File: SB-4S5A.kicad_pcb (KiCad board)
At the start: 4 copper layers, 100 x 50 mm, 41 parts, among them J1 Conn_02x03_Top_Bottom, Q1 CSD17308Q3, Q2 CSD17308Q3, Q3 2N7002, U1 bq40z50-r2

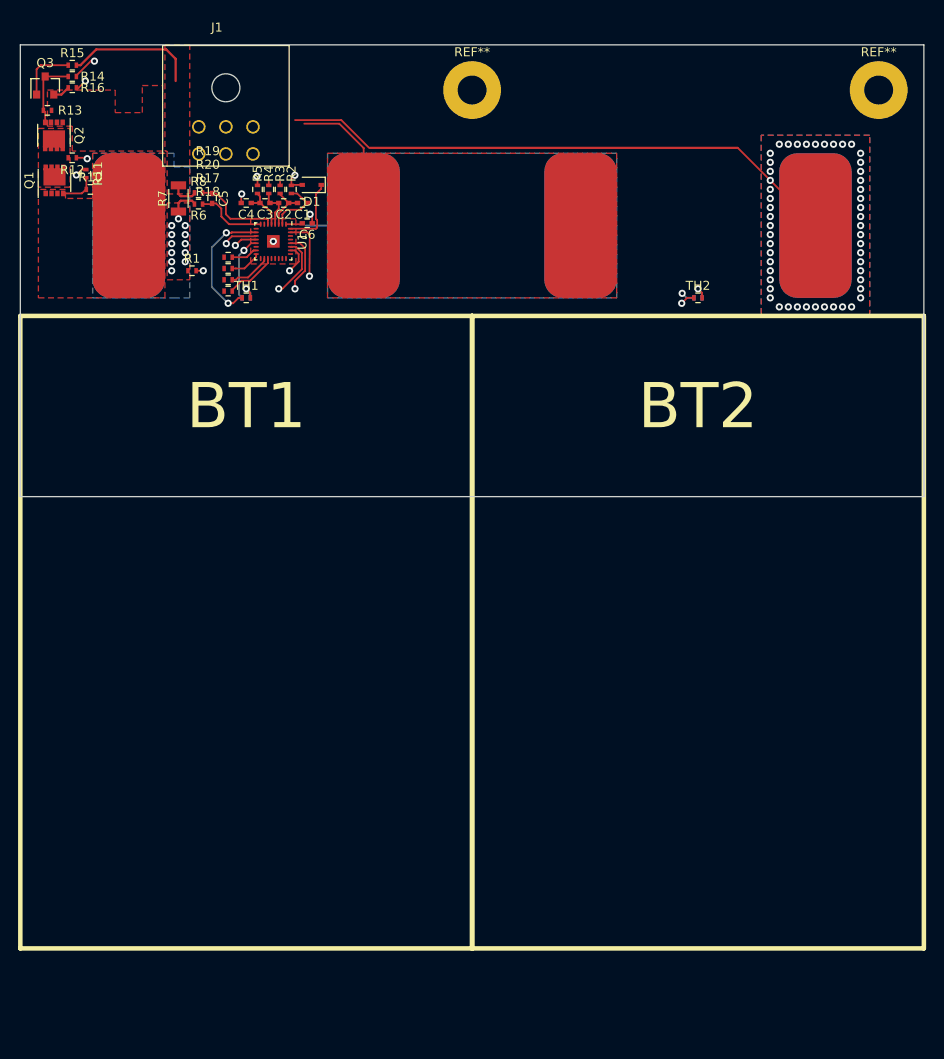
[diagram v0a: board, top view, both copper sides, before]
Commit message: Ready to send to manufacturer.
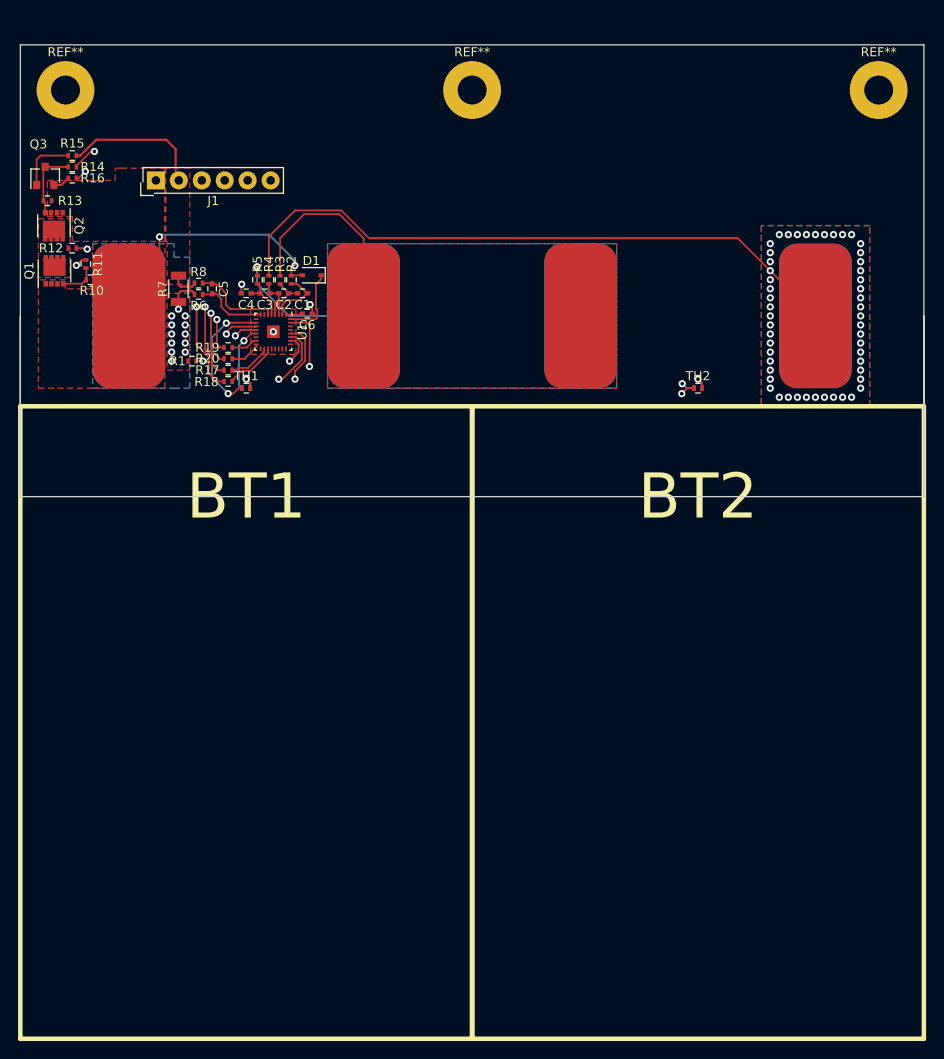
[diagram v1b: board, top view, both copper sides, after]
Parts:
- added REF**: MountingHole_3.2mm_M3_Pad, Mounting_Holes:MountingHole_3.2mm_M3_Pad, F.Cu at (75.0, 65.0)
- J1: value Conn_02x03_Top_Bottom -> LEMO6; footprint Connectors_Molex:Molex_Microfit3_Header_02x03_Angled_43045-060x -> Connectors_Samtec:SL-106-X-XX_1x06
- moved BT1 10.0 mm to (95.0, 100.0)
- moved BT2 10.0 mm to (145.0, 100.0)
- moved BT3 10.0 mm to (145.0, 100.0)
- moved BT4 10.0 mm to (95.0, 100.0)
- moved C1 10.0 mm to (101.2, 87.5)
- moved C2 10.0 mm to (99.2, 87.5)
- moved C3 10.0 mm to (97.1, 87.5)
- moved C4 10.0 mm to (95.0, 87.5)
- moved C5 10.0 mm to (91.2, 87.0)
- moved C6 10.0 mm to (101.8, 89.8)
- moved D1 10.0 mm to (102.2, 85.5)
- moved Q1 10.0 mm to (73.8, 85.0)
- moved Q2 10.0 mm to (73.7, 80.0)
- moved Q3 10.0 mm to (72.8, 74.5)
- moved R1 10.0 mm to (89.0, 95.0)
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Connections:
- U1 pad 17: Net-(U1-Pad17) -> (no net)
- U1 pad 20: Net-(U1-Pad20) -> (no net)
- U1 pad 21: Net-(U1-Pad21) -> (no net)
- U1 pad 22: Net-(U1-Pad22) -> (no net)
- U1 pad 25: Net-(U1-Pad25) -> (no net)
- U1 pad 30: Net-(U1-Pad30) -> (no net)
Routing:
- net /BAT+: track 2.50 -> 29.5 mm, vias 1 -> 2
- net /BTP_INT: track 0.00 -> 24.4 mm, vias 0 -> 1
- net /SMBC: track 0.00 -> 24.2 mm, vias 0 -> 1
- net /~PRES~: track 0.10 -> 23.9 mm, vias 0 -> 1
- net /SMBD: track 0.10 -> 23.3 mm, vias 0 -> 1
- net /VC1A: track 7.42 -> 16.2 mm
- net /VC2A: track 62.9 -> 70.8 mm
- net /VC3A: track 16.7 -> 24.2 mm

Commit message: Fix FUSE pin floating.
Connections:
- U1 pad 25: (no net) -> GNDD
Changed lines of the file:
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@@
   (page A4)
   (layers
-    (0 F.Cu signal hide)
+    (0 F.Cu signal)
     (1 In1.Cu mixed hide)
     (2 In2.Cu mixed hide)
@@
     (pad 24 smd oval (at 1.9 -1.4) (size 0.2 0.6) (layers F.Cu F.Paste F.Mask)
       (net 1 GNDD))
-    (pad 25 smd oval (at 1.4 -1.9 270) (size 0.2 0.6) (layers F.Cu F.Paste F.Mask))
+    (pad 25 smd oval (at 1.4 -1.9 270) (size 0.2 0.6) (layers F.Cu F.Paste F.Mask)
+      (net 1 GNDD))
     (pad 26 smd oval (at 1 -1.9 270) (size 0.2 0.6) (layers F.Cu F.Paste F.Mask)
       (net 30 /_VCC_))
@@
   (segment (start 103.3 85.925) (end 103.3 85.5) (width 0.2) (layer F.Cu) (net 21) (status 20))
   (segment (start 91.2 95.4) (end 91.8 96) (width 0.2) (layer F.Cu) (net 22))
-  (segment (start 91.8 96) (end 92.55 96) (width 0.2) (layer F.Cu) (net 22))
+  (segment (start 91.8 96) (end 92.55 96) (width 0.2) (layer F.Cu) (net 22) (status 20))
   (segment (start 91.2 94.4) (end 91.2 95.4) (width 0.2) (layer F.Cu) (net 22))
   (segment (start 90.45 93.65) (end 91.2 94.4) (width 0.2) (layer F.Cu) (net 22))
   (segment (start 90.45 89) (end 90.45 93.65) (width 0.2) (layer F.Cu) (net 22))
-  (segment (start 92.62 75) (end 90.45 77.17) (width 0.2) (layer In2.Cu) (net 22))
+  (segment (start 92.62 75) (end 90.45 77.17) (width 0.2) (layer In2.Cu) (net 22) (status 10))
   (segment (start 90.45 77.17) (end 90.45 89) (width 0.2) (layer In2.Cu) (net 22))
   (via (at 90.45 89) (size 0.8) (drill 0.4) (layers F.Cu B.Cu) (net 22))
@@
   (segment (start 90.08 88.42) (end 89.5 89) (width 0.2) (layer In2.Cu) (net 23))
   (segment (start 91.1 93.8) (end 92.05 94.75) (width 0.2) (layer F.Cu) (net 24))
-  (segment (start 92.05 94.75) (end 92.55 94.75) (width 0.2) (layer F.Cu) (net 24))
+  (segment (start 92.05 94.75) (end 92.55 94.75) (width 0.2) (layer F.Cu) (net 24) (status 20))
   (segment (start 91.1 89.7) (end 91.1 93.8) (width 0.2) (layer F.Cu) (net 24))
   (segment (start 90.8 88.4) (end 91.1 88.7) (width 0.2) (layer In2.Cu) (net 24))
@@
   (segment (start 91.2 76.95) (end 90.8 77.35) (width 0.2) (layer In2.Cu) (net 24))
   (segment (start 93.21 76.95) (end 91.2 76.95) (width 0.2) (layer In2.Cu) (net 24))
-  (segment (start 95.16 75) (end 93.21 76.95) (width 0.2) (layer In2.Cu) (net 24))
+  (segment (start 95.16 75) (end 93.21 76.95) (width 0.2) (layer In2.Cu) (net 24) (status 10))
   (segment (start 92.55 94.75) (end 92.55 94.65) (width 0.2) (layer F.Cu) (net 24) (status 30))
   (segment (start 91.75 90.4) (end 91.75 93.1) (width 0.2) (layer F.Cu) (net 25))
   (segment (start 91.75 93.1) (end 92.15 93.5) (width 0.2) (layer F.Cu) (net 25))
-  (segment (start 92.15 93.5) (end 92.55 93.5) (width 0.2) (layer F.Cu) (net 25))
+  (segment (start 92.15 93.5) (end 92.55 93.5) (width 0.2) (layer F.Cu) (net 25) (status 20))
   (segment (start 91.15 88.25) (end 91.75 88.85) (width 0.2) (layer In2.Cu) (net 25))
   (segment (start 91.75 88.85) (end 91.75 90.4) (width 0.2) (layer In2.Cu) (net 25))
@@
   (segment (start 91.35 77.3) (end 91.15 77.5) (width 0.2) (layer In2.Cu) (net 25))
   (segment (start 95.4 77.3) (end 91.35 77.3) (width 0.2) (layer In2.Cu) (net 25))
-  (segment (start 97.7 75) (end 95.4 77.3) (width 0.2) (layer In2.Cu) (net 25))
+  (segment (start 97.7 75) (end 95.4 77.3) (width 0.2) (layer In2.Cu) (net 25) (status 10))
   (segment (start 77.3 86) (end 77.3 84.75) (width 0.2) (layer F.Cu) (net 27) (status 30))
   (segment (start 77.3 84.75) (end 77.25 84.7) (width 0.2) (layer F.Cu) (net 27) (status 30))
